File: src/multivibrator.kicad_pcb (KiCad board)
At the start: 2 copper layers, 40.6 x 26.7 mm, 11 parts, among them P1 CONN_01X02, Q1 Q_NPN_EBC, Q2 Q_NPN_EBC

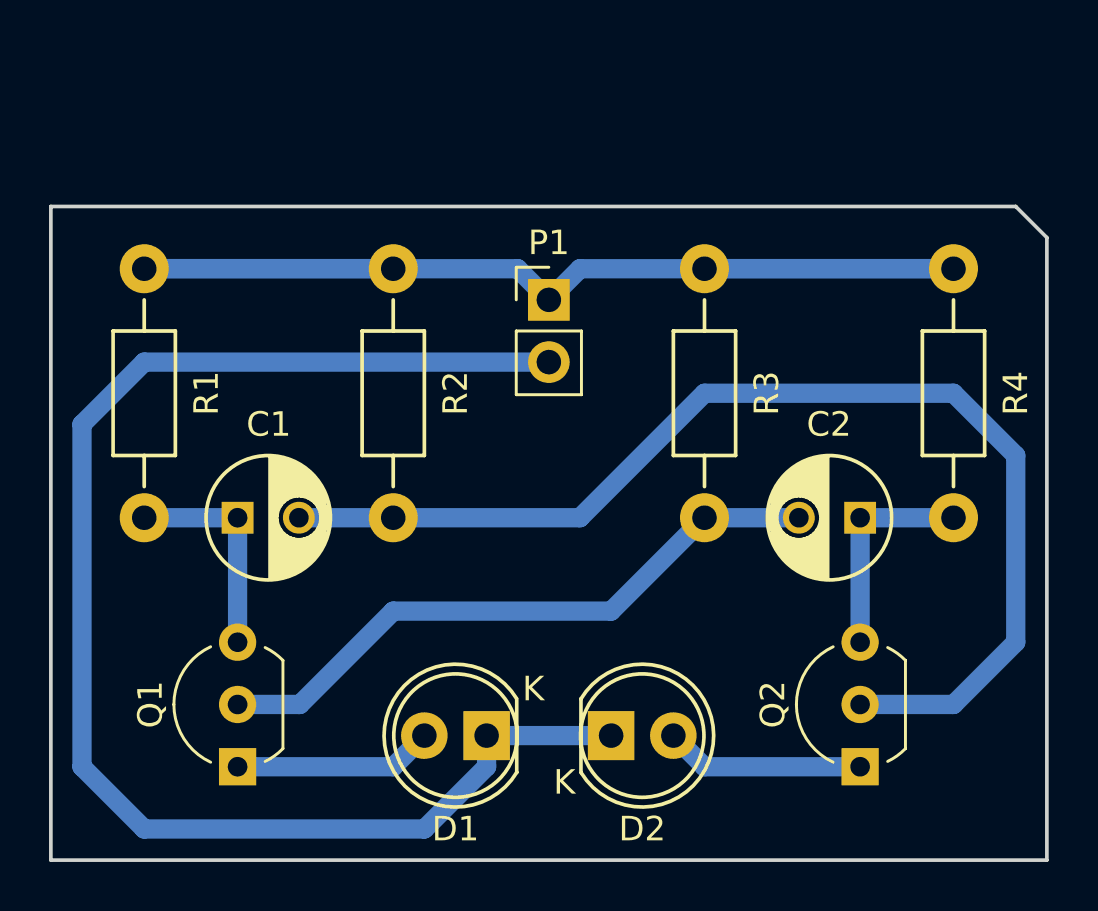
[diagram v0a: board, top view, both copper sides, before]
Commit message: made a smaller pcb?
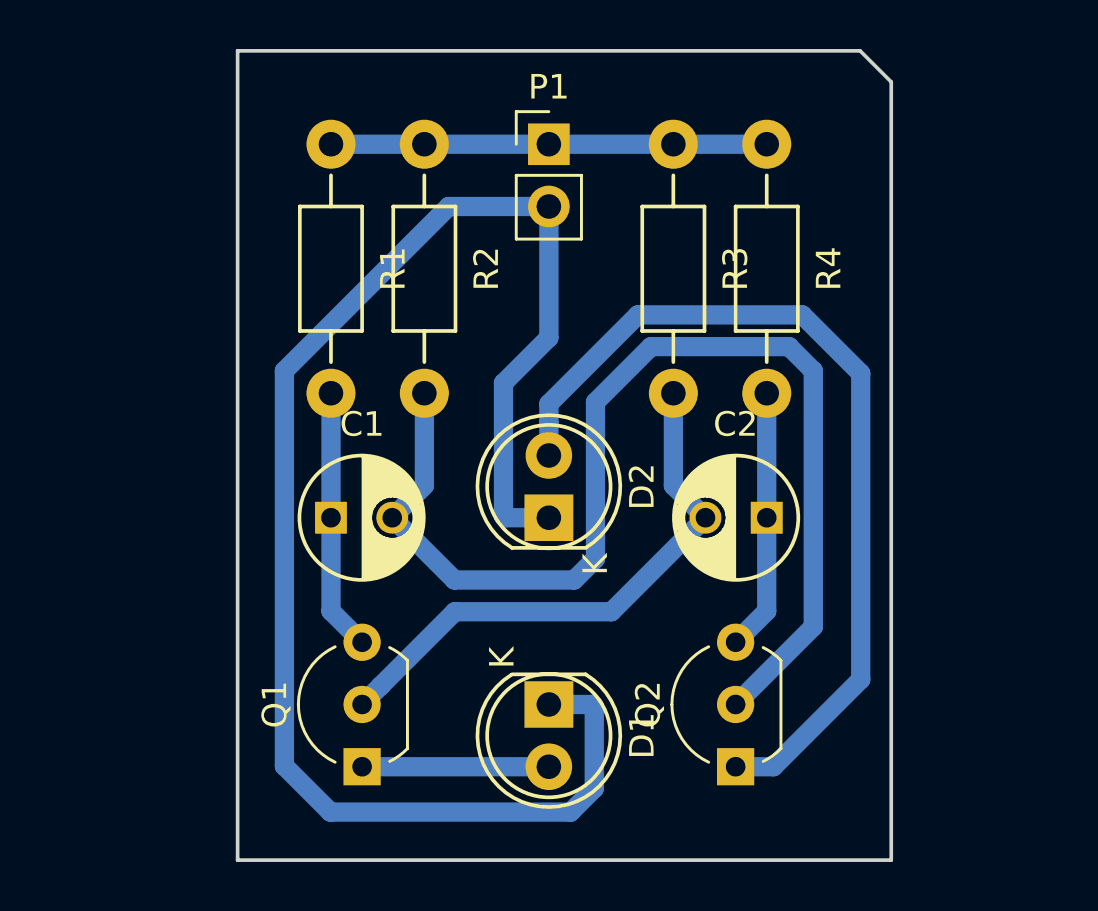
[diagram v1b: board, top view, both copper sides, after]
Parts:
- moved D2 9.25 mm to (99.1, 74.9), turned to 90 degrees
- moved R1 9.16 mm to (90.2, 59.7)
- moved R4 9.16 mm to (108.0, 59.7)
- moved P1 6.35 mm to (99.1, 59.7)
- moved R2 5.24 mm to (94.0, 59.7)
- moved R3 5.24 mm to (104.1, 59.7)
- moved Q1 5.08 mm to (91.4, 85.1)
- moved Q2 5.08 mm to (106.7, 85.1)
- moved C1 3.81 mm to (90.2, 74.9)
- moved C2 3.81 mm to (108.0, 74.9)
- moved D1 2.84 mm to (99.1, 82.5), turned to 270 degrees
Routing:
- net Net-(D2-Pad2): track 8.15 -> 36.4 mm
- net VCC: track 34.1 -> 17.8 mm
- net GND: track 59.0 -> 64.0 mm
- net Net-(C2-Pad2): track 26.1 -> 22.8 mm
- net Net-(C2-Pad1): track 8.89 -> 10.7 mm
- net Net-(C1-Pad1): track 8.89 -> 10.7 mm
- net Net-(C1-Pad2): track 47.4 -> 46.9 mm
- net Net-(D1-Pad2): track 8.15 -> 7.62 mm
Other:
- board size 40.6 x 26.7 mm -> 26.7 x 33 mm
